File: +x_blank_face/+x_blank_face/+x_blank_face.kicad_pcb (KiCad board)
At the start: 2 copper layers, 87 x 326.5 mm, 25 parts, among them J1 Conn_01x08_Pin, J2 Conn_01x02_Pin, J3 Conn_01x02_Pin

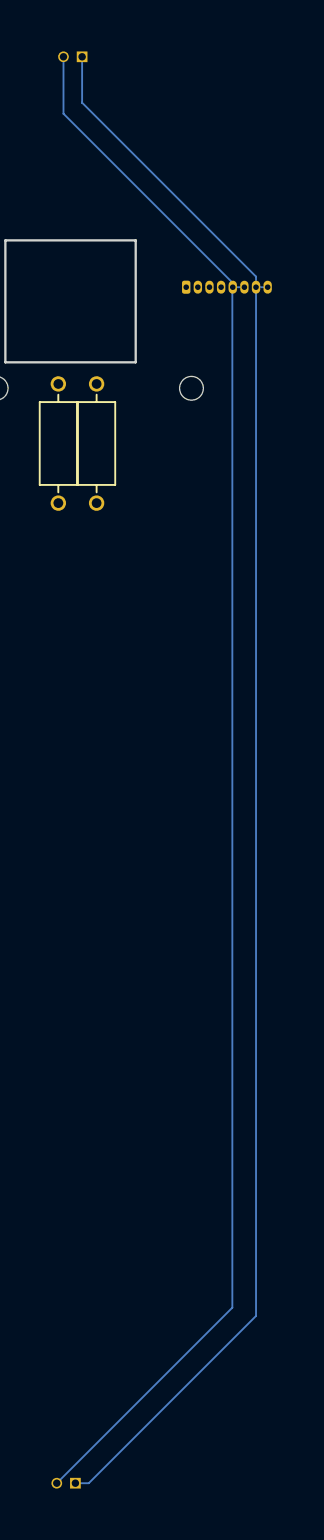
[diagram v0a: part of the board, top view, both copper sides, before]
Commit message: I forgot what I changed
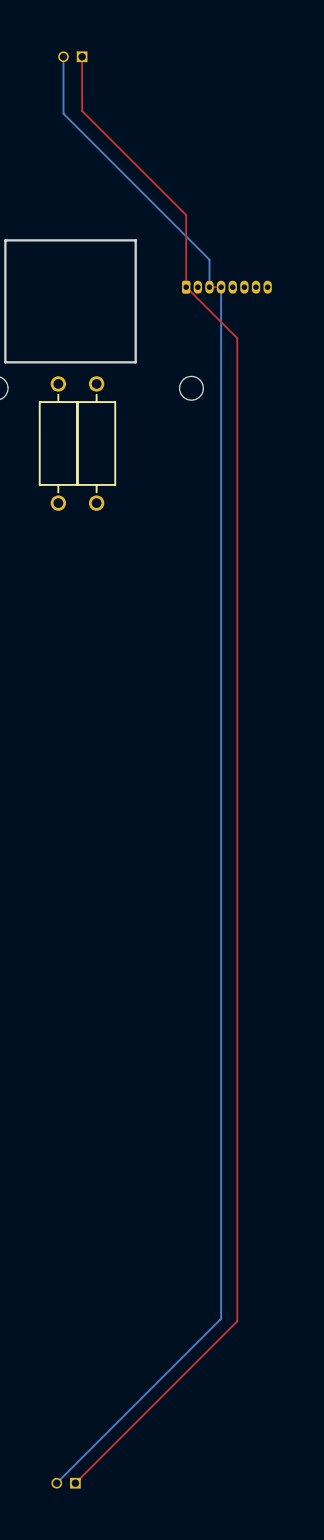
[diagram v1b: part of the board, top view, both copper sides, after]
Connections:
- J1 pad 1: /12VPDM -> GND
- J1 pad 2: /12VPDM -> GND
- J1 pad 3: /+X Drain -> /-X Serial Out
- J1 pad 4: /+X Drain -> /-X Serial Out
- J1 pad 5: /-X Serial Out -> /+X Drain
- J1 pad 6: /-X Serial Out -> /+X Drain
- J1 pad 7: GND -> /12VPDM
- J1 pad 8: GND -> /12VPDM
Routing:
- net GND: track 171.1 -> 167.3 mm
- net /-X Serial Out: track 169.8 -> 168.3 mm
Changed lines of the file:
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@@
 			(remove_unused_layers no)
 			(roundrect_rratio 0.25)
-			(net 1 "/12VPDM")
+			(net 4 "GND")
 			(pinfunction "Pin_1")
 			(pintype "passive")
@@
 			(layers "*.Cu" "*.Mask")
 			(remove_unused_layers no)
-			(net 1 "/12VPDM")
+			(net 4 "GND")
 			(pinfunction "Pin_2")
 			(pintype "passive")
@@
 			(layers "*.Cu" "*.Mask")
 			(remove_unused_layers no)
-			(net 3 "/+X Drain")
+			(net 2 "/-X Serial Out")
 			(pinfunction "Pin_3")
 			(pintype "passive")
@@
 			(layers "*.Cu" "*.Mask")
 			(remove_unused_layers no)
-			(net 3 "/+X Drain")
+			(net 2 "/-X Serial Out")
 			(pinfunction "Pin_4")
 			(pintype "passive")
@@
 			(layers "*.Cu" "*.Mask")
 			(remove_unused_layers no)
-			(net 2 "/-X Serial Out")
+			(net 3 "/+X Drain")
 			(pinfunction "Pin_5")
 			(pintype "passive")
@@
 			(layers "*.Cu" "*.Mask")
 			(remove_unused_layers no)
-			(net 2 "/-X Serial Out")
+			(net 3 "/+X Drain")
 			(pinfunction "Pin_6")
 			(pintype "passive")
@@
 			(layers "*.Cu" "*.Mask")
 			(remove_unused_layers no)
-			(net 4 "GND")
+			(net 1 "/12VPDM")
 			(pinfunction "Pin_7")
 			(pintype "passive")
@@
 			(layers "*.Cu" "*.Mask")
 			(remove_unused_layers no)
-			(net 4 "GND")
+			(net 1 "/12VPDM")
 			(pinfunction "Pin_8")
 			(pintype "passive")
@@
 	)
 	(segment
-		(start 173.0325 149.65)
-		(end 191.89 130.7925)
+		(start 189.435 21.18)
+		(end 190.685 21.18)
+		(width 0.2)
+		(layer "F.Cu")
+		(net 2)
+	)
+	(segment
+		(start 173.0325 149.6375)
+		(end 190.585 132.085)
 		(width 0.2)
 		(layer "B.Cu")
@@
 	)
 	(segment
+		(start 190.685 131.985)
+		(end 190.585 132.085)
+		(width 0.2)
+		(layer "B.Cu")
+		(net 2)
+	)
+	(segment
+		(start 189.435 18.227926)
+		(end 189.435 21.18)
+		(width 0.2)
+		(layer "B.Cu")
+		(net 2)
+	)
+	(segment
 		(start 173.7525 -3.57)
 		(end 173.7525 2.545426)
@@
 	)
 	(segment
-		(start 191.935 21.18)
-		(end 193.185 21.18)
+		(start 173.7525 2.545426)
+		(end 189.435 18.227926)
 		(width 0.2)
 		(layer "B.Cu")
@@
 	)
 	(segment
-		(start 191.89 130.7925)
-		(end 191.89 21.655)
+		(start 190.685 21.18)
+		(end 190.685 131.985)
 		(width 0.2)
 		(layer "B.Cu")
@@
 	)
 	(segment
-		(start 191.935 20.727926)
-		(end 173.7525 2.545426)
+		(start 173.0325 149.65)
+		(end 173.0325 149.6375)
 		(width 0.2)
 		(layer "B.Cu")
@@
 	(segment
 		(start 191.935 21.18)
-		(end 191.935 20.727926)
+		(end 191.935 21.61)
 		(width 0.2)
 		(layer "B.Cu")
-		(net 2)
-	)
-	(segment
-		(start 191.935 21.18)
-		(end 191.935 21.61)
-		(width 0.2)
-		(layer "B.Cu")
-		(net 2)
+		(net 3)
 	)
 	(segment
@@
 		(width 0.2)
 		(layer "B.Cu")
-		(net 2)
-	)
-	(segment
-		(start 194.435 21.18)
-		(end 195.685 21.18)
-		(width 0.2)
-		(layer "B.Cu")
+		(net 3)
+	)
+	(segment
+		(start 192.42 132.2625)
+		(end 192.42 26.665)
+		(width 0.2)
+		(layer "F.Cu")
 		(net 4)
 	)
 	(segment
-		(start 175.75 1.36)
-		(end 194.435 20.045)
-		(width 0.2)
-		(layer "B.Cu")
+		(start 192.42 26.665)
+		(end 186.935 21.18)
+		(width 0.2)
+		(layer "F.Cu")
 		(net 4)
 	)
 	(segment
-		(start 176.47 149.65)
-		(end 194.435 131.685)
-		(width 0.2)
-		(layer "B.Cu")
+		(start 175.7525 -3.57)
+		(end 175.7525 2.2525)
+		(width 0.2)
+		(layer "F.Cu")
 		(net 4)
 	)
 	(segment
-		(start 194.435 21.18)
-		(end 194.435 131.685)
-		(width 0.2)
-		(layer "B.Cu")
+		(start 175.7525 2.2525)
+		(end 186.935 13.435)
+		(width 0.2)
+		(layer "F.Cu")
 		(net 4)
 	)
 	(segment
-		(start 175.7525 -3.57)
-		(end 175.7525 1.3575)
-		(width 0.2)
-		(layer "B.Cu")
+		(start 186.935 13.435)
+		(end 186.935 21.18)
+		(width 0.2)
+		(layer "F.Cu")
 		(net 4)
 	)
 	(segment
-		(start 175.7525 1.3575)
-		(end 175.75 1.36)
-		(width 0.2)
-		(layer "B.Cu")
+		(start 175.0325 149.65)
+		(end 192.42 132.2625)
+		(width 0.2)
+		(layer "F.Cu")
 		(net 4)
 	)
-	(segment
-		(start 175.0325 149.65)
-		(end 176.47 149.65)
-		(width 0.2)
-		(layer "B.Cu")
-		(net 4)
-	)
-	(segment
-		(start 194.435 20.045)
-		(end 194.435 21.18)
-		(width 0.2)
-		(layer "B.Cu")
-		(net 4)
-	)

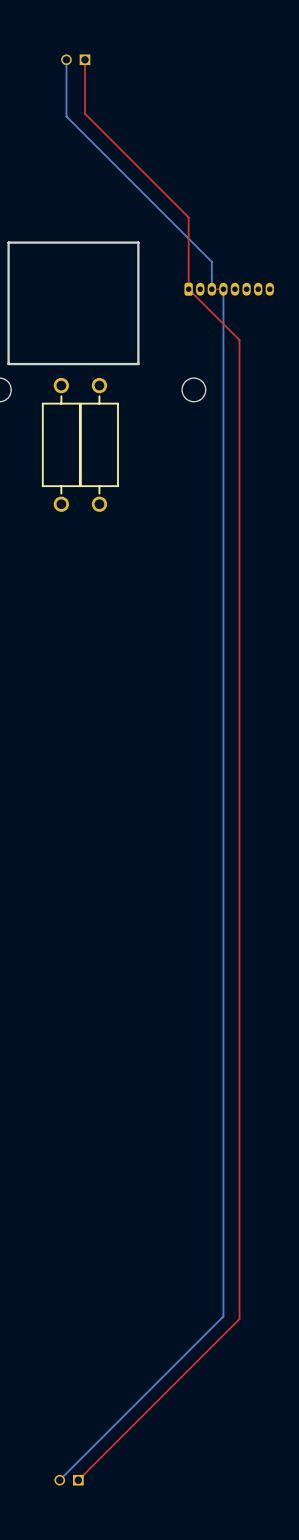
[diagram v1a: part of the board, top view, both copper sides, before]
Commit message: Rerouted some stuff
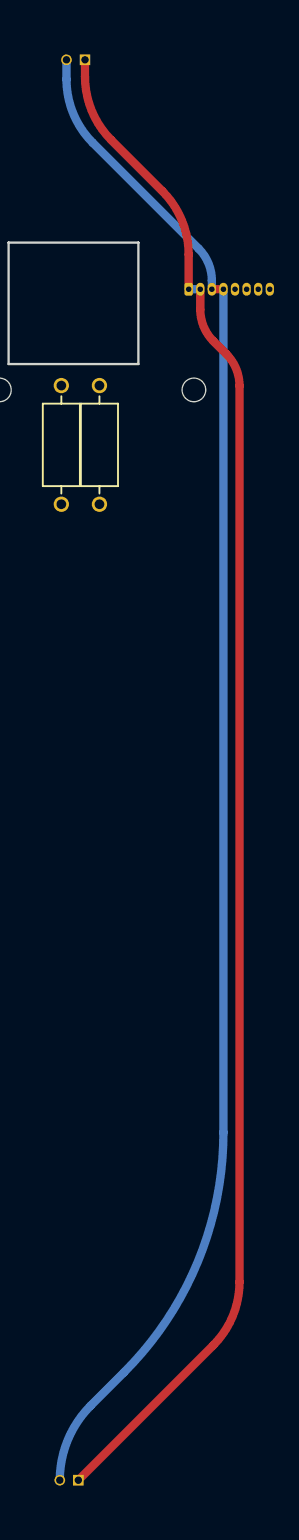
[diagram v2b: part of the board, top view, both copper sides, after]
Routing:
- net /-X Serial Out: track 168.3 -> 165.3 mm
- net GND: track 167.3 -> 166.2 mm
